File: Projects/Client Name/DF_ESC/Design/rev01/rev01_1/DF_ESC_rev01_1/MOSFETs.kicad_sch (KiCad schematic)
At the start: 34 parts, among them J5 7461084, J6 7461084, J7 7461084, Q1 HSBA15810C, Q2 HSBA15810C, Q3 HSBA15810C, Q4 HSBA15810C, Q5 HSBA15810C, Q6 HSBA15810C

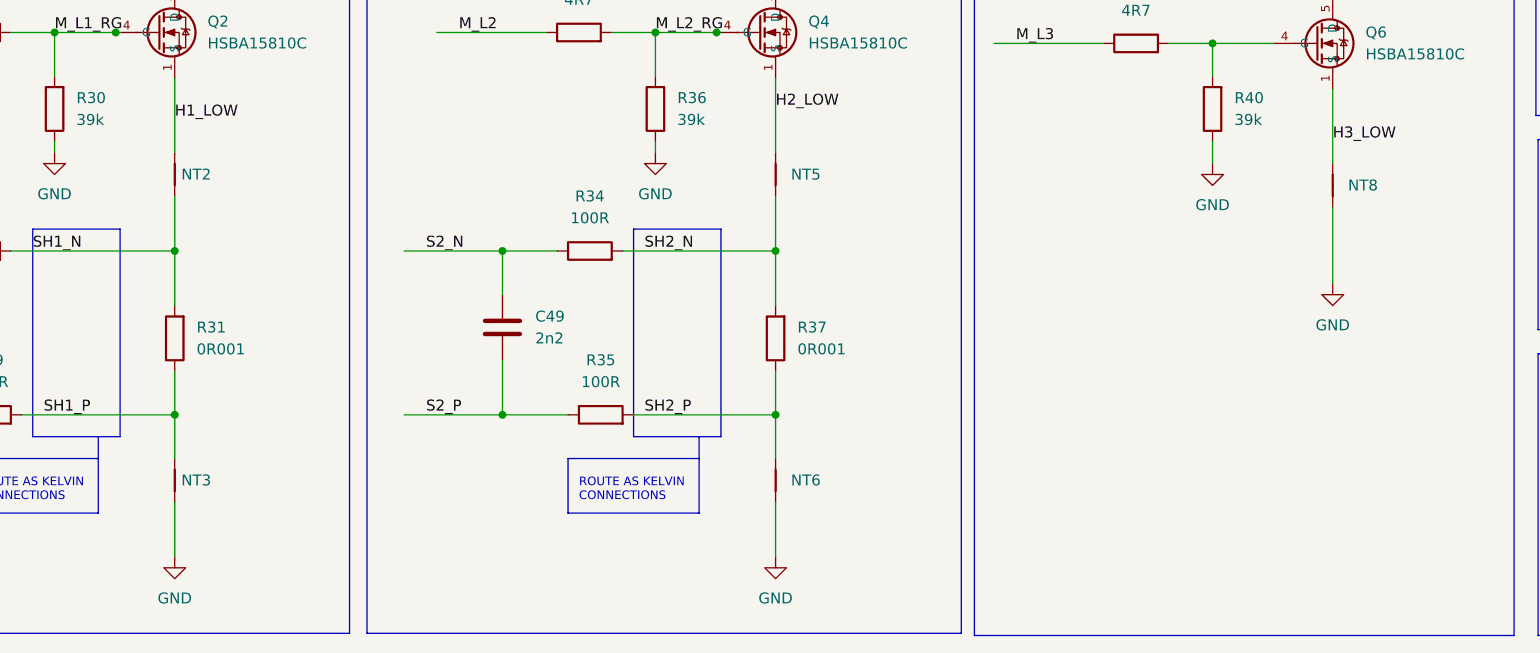
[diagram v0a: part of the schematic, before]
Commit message: Update 2024-03-13_2
Version final para posicionar PCB
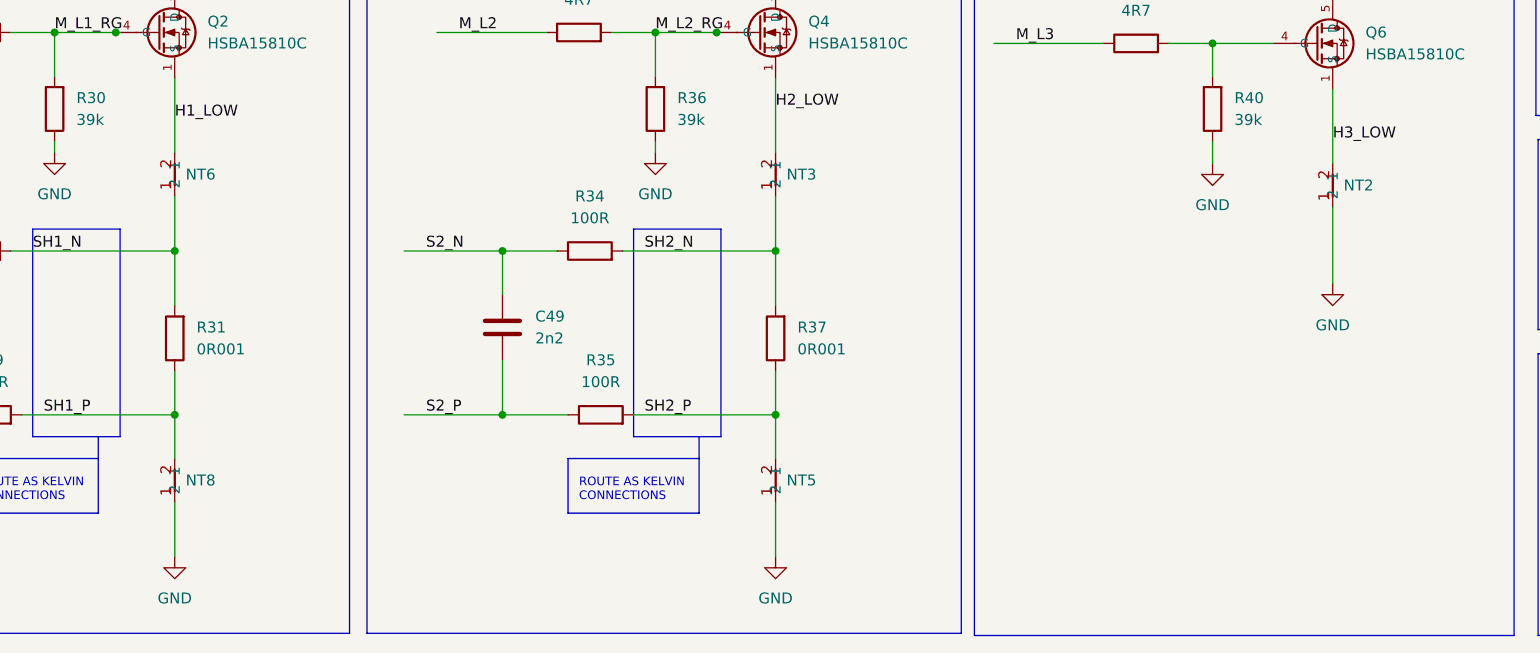
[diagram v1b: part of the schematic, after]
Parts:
- removed NT2, NT5, NT8: NetTie_2, symbol Device:NetTie_2
- removed NT3, NT6: ~, symbol Device:NetTie_2
- added NT2, NT3, NT5, NT6, NT8: Net_Tie_PWR, DF_ESC_Footprint_Library:NetTie_SMD_Pad_3.00mm, symbol DF_ESC_Symbol_Library:Net_Tie_PWR
- NT1, NT4, NT7: footprint (none) -> NetTie:NetTie-2_SMD_Pad0.5mm
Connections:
- net GND: now also NT2.1, NT5.1, NT8.1
- net H1_LOW: now also NT6.2
- net H2_LOW: now also NT3.2
- net H3_LOW: now also NT2.2
- net SH1_N: now also NT6.1
- net SH1_P: now also NT8.2
- net SH2_N: now also NT3.1
- net SH2_P: now also NT5.2

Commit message: update 07-04-2024
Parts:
- R31, R37: footprint Resistor_SMD:R_0603_1608Metric_Pad0.98x0.95mm_HandSolder -> DF_ESC_Footprint_Library:RES-SMD_L7.0-W6.7
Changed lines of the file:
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@@
 			)
 		)
-		(property "Footprint" "Resistor_SMD:R_0603_1608Metric_Pad0.98x0.95mm_HandSolder"
+		(property "Footprint" "DF_ESC_Footprint_Library:RES-SMD_L7.0-W6.7"
 			(at 97.028 128.27 90)
 			(effects
@@
 			)
 		)
-		(property "Footprint" "Resistor_SMD:R_0603_1608Metric_Pad0.98x0.95mm_HandSolder"
+		(property "Footprint" "DF_ESC_Footprint_Library:RES-SMD_L7.0-W6.7"
 			(at 166.878 128.27 90)
 			(effects

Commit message: update 20240427
Mejora de layout cero errores, solo falta añadir algunas reseñas en el silkscreen
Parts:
- Q1, Q2, Q3, Q4, Q5, Q6: footprint DF_ESC_Footprint_Library_Casa:PQFN-8_L6.0-W5.0-P1.27-LS6.0-BL -> DF_ESC_Footprint_Library:PQFN-8_L6.0-W5.0-P1.27-LS6.0-BL
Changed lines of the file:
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@@
 			)
 		)
-		(property "Footprint" "DF_ESC_Footprint_Library_Casa:PQFN-8_L6.0-W5.0-P1.27-LS6.0-BL"
+		(property "Footprint" "DF_ESC_Footprint_Library:PQFN-8_L6.0-W5.0-P1.27-LS6.0-BL"
 			(at 169.418 62.484 0)
 			(effects
@@
 			)
 		)
-		(property "Footprint" "DF_ESC_Footprint_Library_Casa:PQFN-8_L6.0-W5.0-P1.27-LS6.0-BL"
+		(property "Footprint" "DF_ESC_Footprint_Library:PQFN-8_L6.0-W5.0-P1.27-LS6.0-BL"
 			(at 99.568 87.884 0)
 			(effects
@@
 			)
 		)
-		(property "Footprint" "DF_ESC_Footprint_Library_Casa:PQFN-8_L6.0-W5.0-P1.27-LS6.0-BL"
+		(property "Footprint" "DF_ESC_Footprint_Library:PQFN-8_L6.0-W5.0-P1.27-LS6.0-BL"
 			(at 234.188 62.484 0)
 			(effects
@@
 			)
 		)
-		(property "Footprint" "DF_ESC_Footprint_Library_Casa:PQFN-8_L6.0-W5.0-P1.27-LS6.0-BL"
+		(property "Footprint" "DF_ESC_Footprint_Library:PQFN-8_L6.0-W5.0-P1.27-LS6.0-BL"
 			(at 99.568 62.484 0)
 			(effects
@@
 			)
 		)
-		(property "Footprint" "DF_ESC_Footprint_Library_Casa:PQFN-8_L6.0-W5.0-P1.27-LS6.0-BL"
+		(property "Footprint" "DF_ESC_Footprint_Library:PQFN-8_L6.0-W5.0-P1.27-LS6.0-BL"
 			(at 169.418 87.884 0)
 			(effects
@@
 			)
 		)
-		(property "Footprint" "DF_ESC_Footprint_Library_Casa:PQFN-8_L6.0-W5.0-P1.27-LS6.0-BL"
+		(property "Footprint" "DF_ESC_Footprint_Library:PQFN-8_L6.0-W5.0-P1.27-LS6.0-BL"
 			(at 234.188 89.154 0)
 			(effects
